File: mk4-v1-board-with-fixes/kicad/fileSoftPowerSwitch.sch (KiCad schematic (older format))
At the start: 12 parts, among them Q2 2N3904, Q26 Q_NMOS_GDS, Q3 2N3904, Q4 2N3904

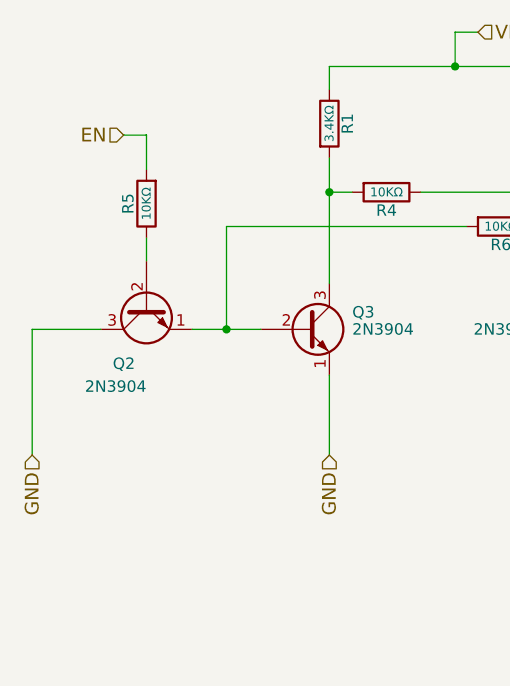
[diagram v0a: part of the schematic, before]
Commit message: Soft push of v2 board modifications
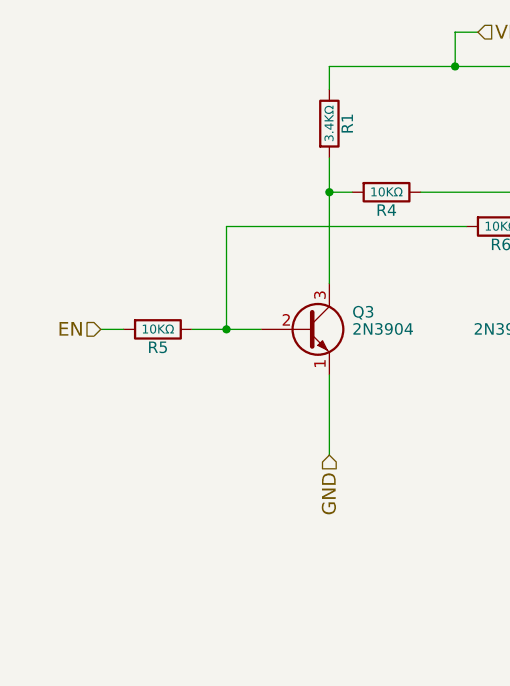
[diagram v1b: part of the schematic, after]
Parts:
- removed Q2: 2N3904, TO_SOT_Packages_THT:TO-92_Molded_Narrow, symbol 2N3904
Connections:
- net at Q3.2 (B), R6.2: now also R5.1
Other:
- moved on the sheet: R5
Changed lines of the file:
@@
 LIBS:valves
 LIBS:freetronics_schematic
+LIBS:cd4013b
 LIBS:hitchco-mk4-cache
 EELAYER 25 0
@@
 $Descr A4 11693 8268
 encoding utf-8
-Sheet 47 47
+Sheet 47 45
 Title ""
 Date ""
@@
 Text HLabel 4400 4200 3    60   Input ~ 0
 GND
-$Comp
-L 2N3904 Q2
-U 1 1 5A25E309
-P 3600 3550
-F 0 "Q2" V 3850 3600 50  0000 L CNN
-F 1 "2N3904" V 3950 3550 50  0000 L CNN
-F 2 "TO_SOT_Packages_THT:TO-92_Molded_Narrow" H 3800 3475 50  0001 L CIN
-F 3 "" H 3600 3550 50  0001 L CNN
-	1    3600 3550
-	0    -1   1    0
-$EndComp
-Text HLabel 3100 4200 3    60   Input ~ 0
-GND
 Text HLabel 5050 2350 2    60   Input ~ 0
 VIN(12V)
@@
 L R R5
 U 1 1 5A25E339
-P 3600 3100
-F 0 "R5" V 3680 3100 50  0000 C CNN
-F 1 "10KΩ" V 3600 3100 39  0000 C CNN
-F 2 "Resistors_THT:R_Axial_DIN0207_L6.3mm_D2.5mm_P10.16mm_Horizontal" V 3530 3100 50  0001 C CNN
-F 3 "" H 3600 3100 50  0001 C CNN
-	1    3600 3100
-	-1   0    0    1
+P 3650 3650
+F 0 "R5" V 3730 3650 50  0000 C CNN
+F 1 "10KΩ" V 3650 3650 39  0000 C CNN
+F 2 "Resistors_THT:R_Axial_DIN0207_L6.3mm_D2.5mm_P10.16mm_Horizontal" V 3580 3650 50  0001 C CNN
+F 3 "" H 3650 3650 50  0001 C CNN
+	1    3650 3650
+	0    1    1    0
 $EndComp
 Wire Wire Line
@@
 Wire Wire Line
 	3950 3200 3950 3650
-Wire Wire Line
-	3800 3650 4100 3650
 Connection ~ 5400 3200
 Wire Wire Line
@@
 	4400 3850 4400 4200
 Connection ~ 3950 3650
-Wire Wire Line
-	3100 3650 3100 4200
-Wire Wire Line
-	3100 3650 3400 3650
 Wire Wire Line
 	4400 2600 4400 2500
@@
 	8350 2350 8200 2350
 Wire Wire Line
-	3600 3250 3600 3350
-Wire Wire Line
-	3500 2800 3600 2800
-Wire Wire Line
-	3600 2800 3600 2950
-Wire Wire Line
 	4950 2350 5050 2350
 Text HLabel 6800 4200 2    60   Input ~ 0
 IS_EN
-Text HLabel 3500 2800 0    60   Input ~ 0
+Text HLabel 3400 3650 0    60   Input ~ 0
 EN
 NoConn ~ 4250 6250
@@
 	1    0    0    -1
 $EndComp
+Wire Wire Line
+	3400 3650 3500 3650
+Wire Wire Line
+	3800 3650 4100 3650
 $EndSCHEMATC
